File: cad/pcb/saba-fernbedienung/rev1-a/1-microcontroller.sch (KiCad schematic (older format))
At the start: 10 parts, among them J201 Conn_ARM_JTAG_SWD_10, Q201 BC856, U201 DOIT-DEVKITV1-ESP32-WROOM-32

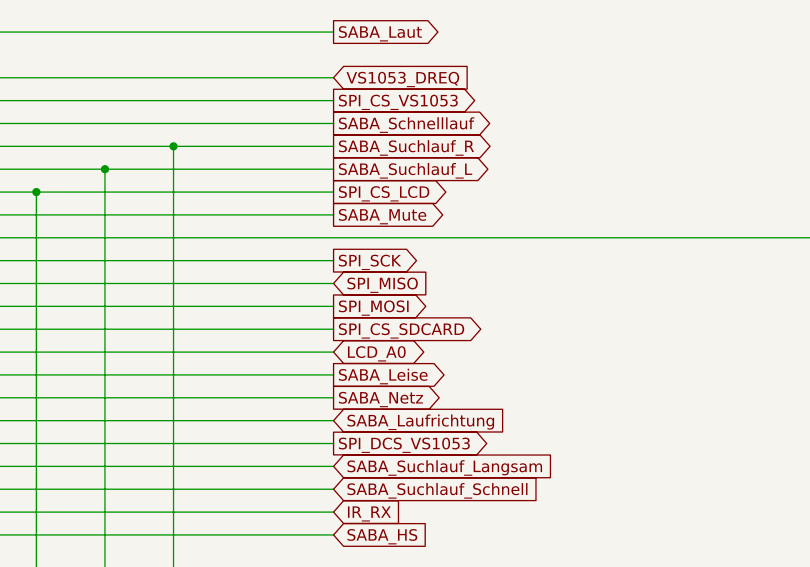
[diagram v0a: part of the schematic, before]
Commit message: Sicherung
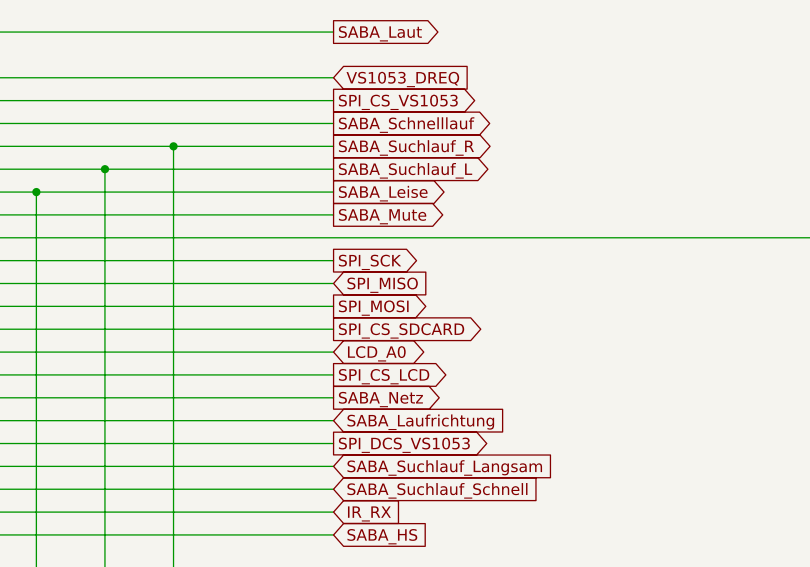
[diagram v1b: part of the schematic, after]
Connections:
- net SABA_Leise: now also R206.2, U201.3 (IO15); no longer U201.23 (IO25)
- net SPI_CS_LCD: now also U201.23 (IO25); no longer R206.2, U201.3 (IO15)
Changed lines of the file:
@@
 Text GLabel 5550 3300 2    50   BiDi ~ 0
 LCD_A0
-Text GLabel 5550 2600 2    50   Output ~ 0
+Text GLabel 5550 3400 2    50   Output ~ 0
 SPI_CS_LCD
 Text GLabel 5550 3200 2    50   Output ~ 0
@@
 Text GLabel 5550 1900 2    50   Output ~ 0
 SABA_Laut
-Text GLabel 5550 3400 2    50   Output ~ 0
+Text GLabel 5550 2600 2    50   Output ~ 0
 SABA_Leise
 Text GLabel 5550 3500 2    50   Output ~ 0
